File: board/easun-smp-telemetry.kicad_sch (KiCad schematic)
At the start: 17 parts, among them J1 INVERTER, J2 PROG, U1 LM1117-3.3, U2 ESP32-C3-WROOM-02, U3 MAX3232 (SP3232E)

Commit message: WIP
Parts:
- U2: footprint Espressif:ESP32-C3-WROOM-02 -> Drake:ESP32-C3-WROOM-02 Handsolder
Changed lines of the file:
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@@
       (effects (font (size 1.27 1.27)))
     )
-    (property "Footprint" "Espressif:ESP32-C3-WROOM-02" (at 152.4 92.71 0)
+    (property "Footprint" "Drake:ESP32-C3-WROOM-02 Handsolder" (at 152.4 92.71 0)
       (effects (font (size 1.27 1.27)) hide)
     )

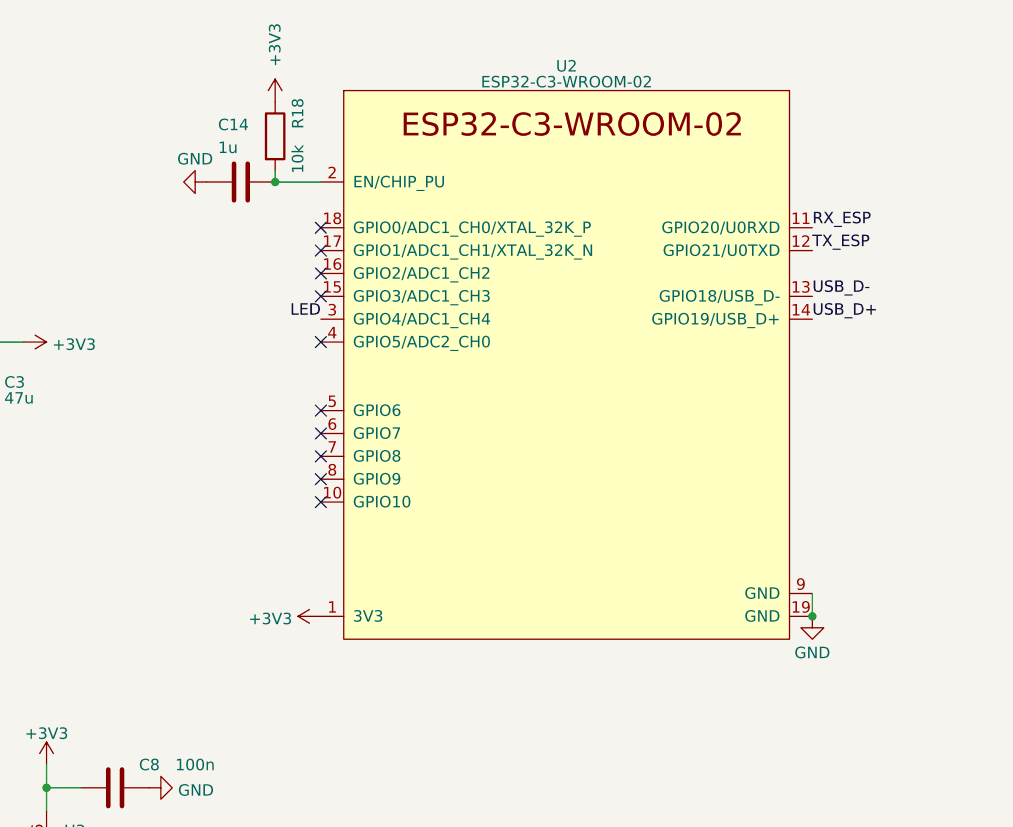
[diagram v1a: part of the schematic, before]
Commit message: library update
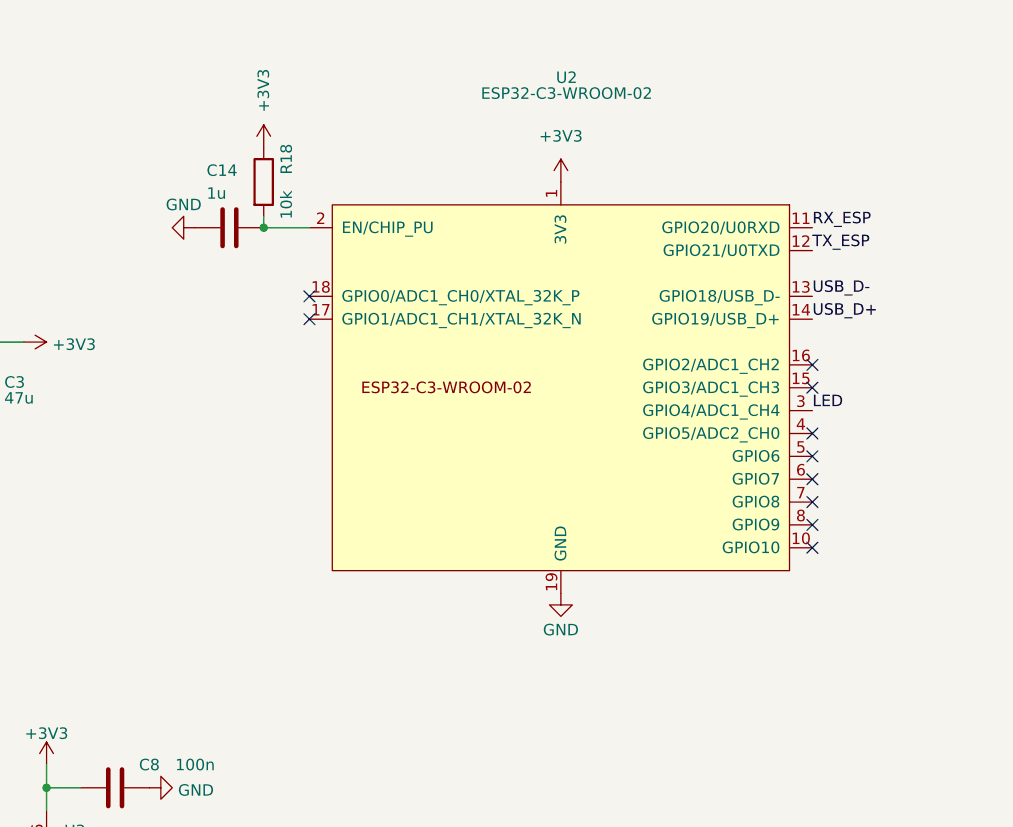
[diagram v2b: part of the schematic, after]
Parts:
- U2: footprint Drake:ESP32-C3-WROOM-02 Handsolder -> PCM_Espressif:ESP32-C3-WROOM-02
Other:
- moved on the sheet: C14, R18
